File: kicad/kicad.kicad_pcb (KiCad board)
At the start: 4 copper layers, 245.1 x 125.7 mm, 31 parts, among them J1 Data In, J2 Power, J3 Address Out, J4 Data Out, J5 Mode Out, SW1 SW_Push_Dual, U1 74LS374, U10 AS6C62256-70PCN, U11 SN74LS682N, U12 74LS374, U13 AT28C256-15PU, U14 SN74HC32N, U15 74LS374, U16 SN74LS682N, U17 SN74HC32N, U18 SN74154N, U2 74LS374, U3 SN74LS04N, U4 W65C02SxP, U5 74LS374, U6 74LS374, U7 SN74LS08N, U8 74LS374, U9 74LS374, X1 CXO_DIP14

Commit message: Save progress on PCB.
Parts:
- moved R4 42.0 mm to (134.6, 61.6)
- moved R2 41.2 mm to (109.9, 73.0), turned to 270 degrees
- moved R3 35.5 mm to (137.2, 83.8)
- moved R1 29.6 mm to (117.5, 83.2), turned to 90 degrees
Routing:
- net Net-(R2-Pad2): track 0.00 -> 30.0 mm
- net Net-(U4-Pad37): track 0.00 -> 18.1 mm
- net Net-(R1-Pad1): track 0.00 -> 10.8 mm
- net Net-(R3-Pad1): track 0.00 -> 3.81 mm
- net Net-(R4-Pad1): track 0.00 -> 3.17 mm
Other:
- board size 245.1 x 125.7 mm -> 165.7 x 93.3 mm
- board text added: "5V"
- board text added: "G"
- board text added: "GND"

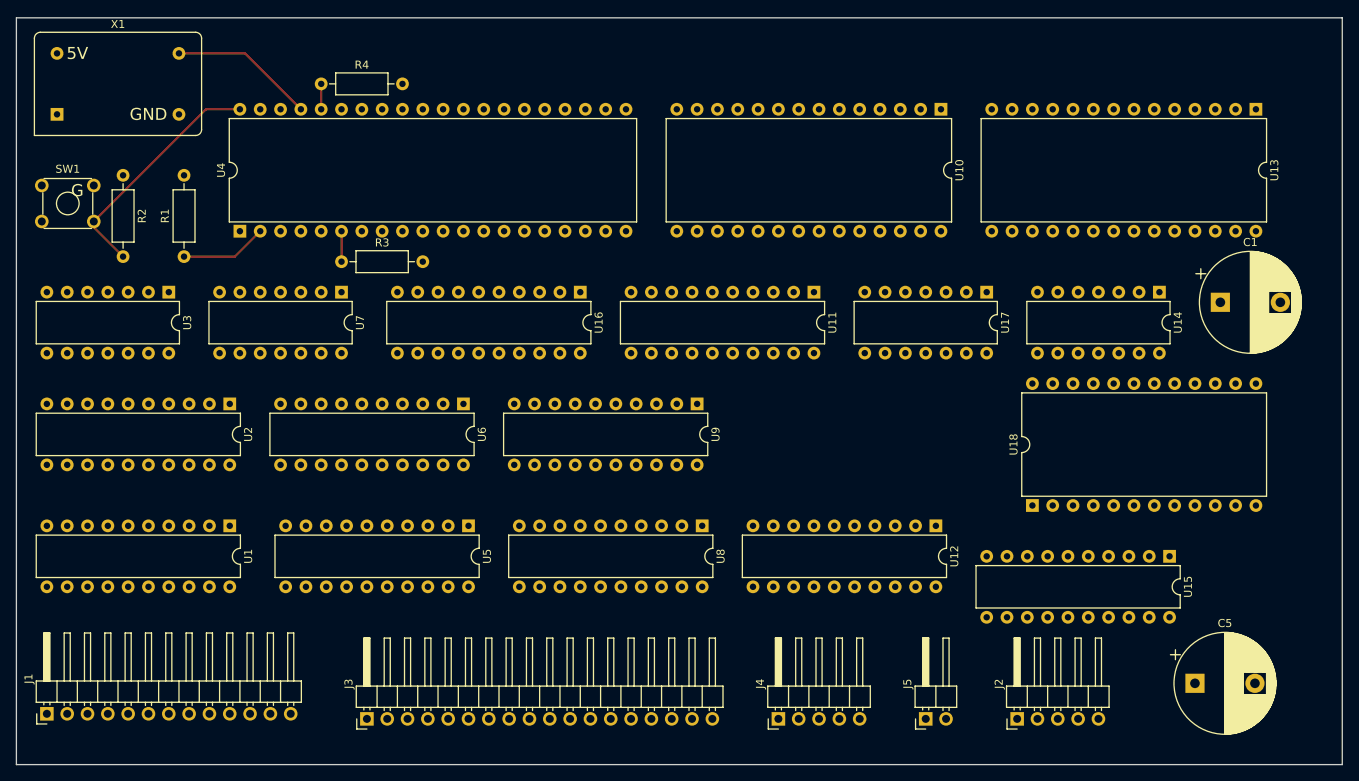
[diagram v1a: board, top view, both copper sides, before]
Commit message: Save progress on PCB.
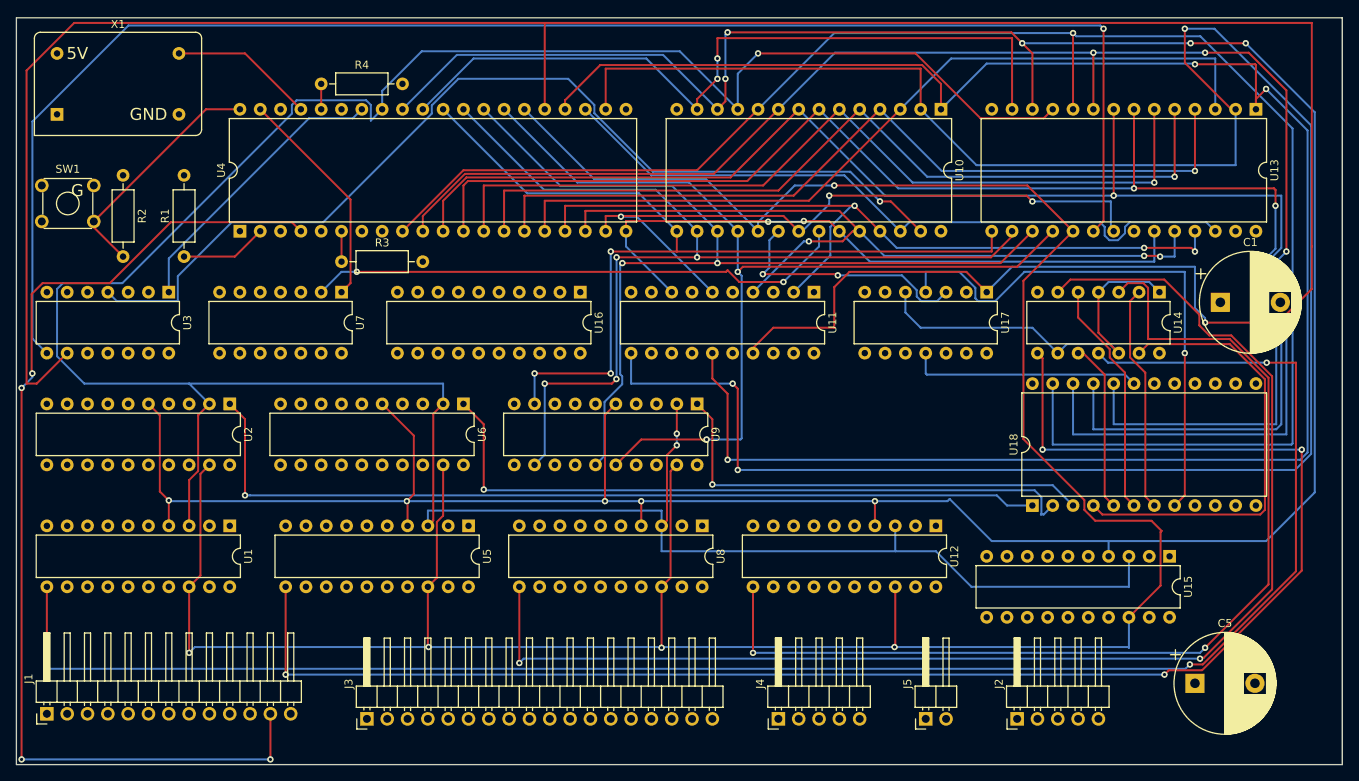
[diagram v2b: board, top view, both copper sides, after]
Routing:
- net Net-(U1-Pad4): track 0.00 -> 391.4 mm, vias 0 -> 10
- net Net-(U1-Pad3): track 0.00 -> 370.3 mm, vias 0 -> 3
- net Net-(U1-Pad18): track 0.00 -> 345.1 mm, vias 0 -> 5
- net Net-(U11-Pad17): track 0.00 -> 340.7 mm, vias 0 -> 1
- net Net-(U10-Pad2): track 0.00 -> 273.7 mm, vias 0 -> 3
- net Net-(U10-Pad1): track 0.00 -> 239.1 mm, vias 0 -> 3
- net Net-(U1-Pad11): track 0.00 -> 222.6 mm, vias 0 -> 3
- net Net-(U10-Pad10): track 0.00 -> 213.0 mm, vias 0 -> 1
- net Net-(U10-Pad9): track 0.00 -> 205.2 mm, vias 0 -> 3
- net Net-(U14-Pad8): track 0.00 -> 203.2 mm, vias 0 -> 4
- net Net-(U13-Pad20): track 0.00 -> 194.6 mm, vias 0 -> 1
- net Net-(U10-Pad8): track 0.00 -> 188.4 mm, vias 0 -> 1
- net Net-(U10-Pad7): track 0.00 -> 181.5 mm, vias 0 -> 2
- net Net-(U14-Pad6): track 0.00 -> 167.3 mm, vias 0 -> 2
- net Net-(J1-Pad12): track 0.00 -> 133.4 mm, vias 0 -> 4
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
